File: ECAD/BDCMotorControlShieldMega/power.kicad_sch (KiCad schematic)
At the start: 15 parts, among them Q1 Q_PMOS, Q2 Q_PMOS, Q3 Q_NMOS, Q4 Q_NMOS, Q5 Q_PNP, Q6 Q_PNP, U33 LM2776

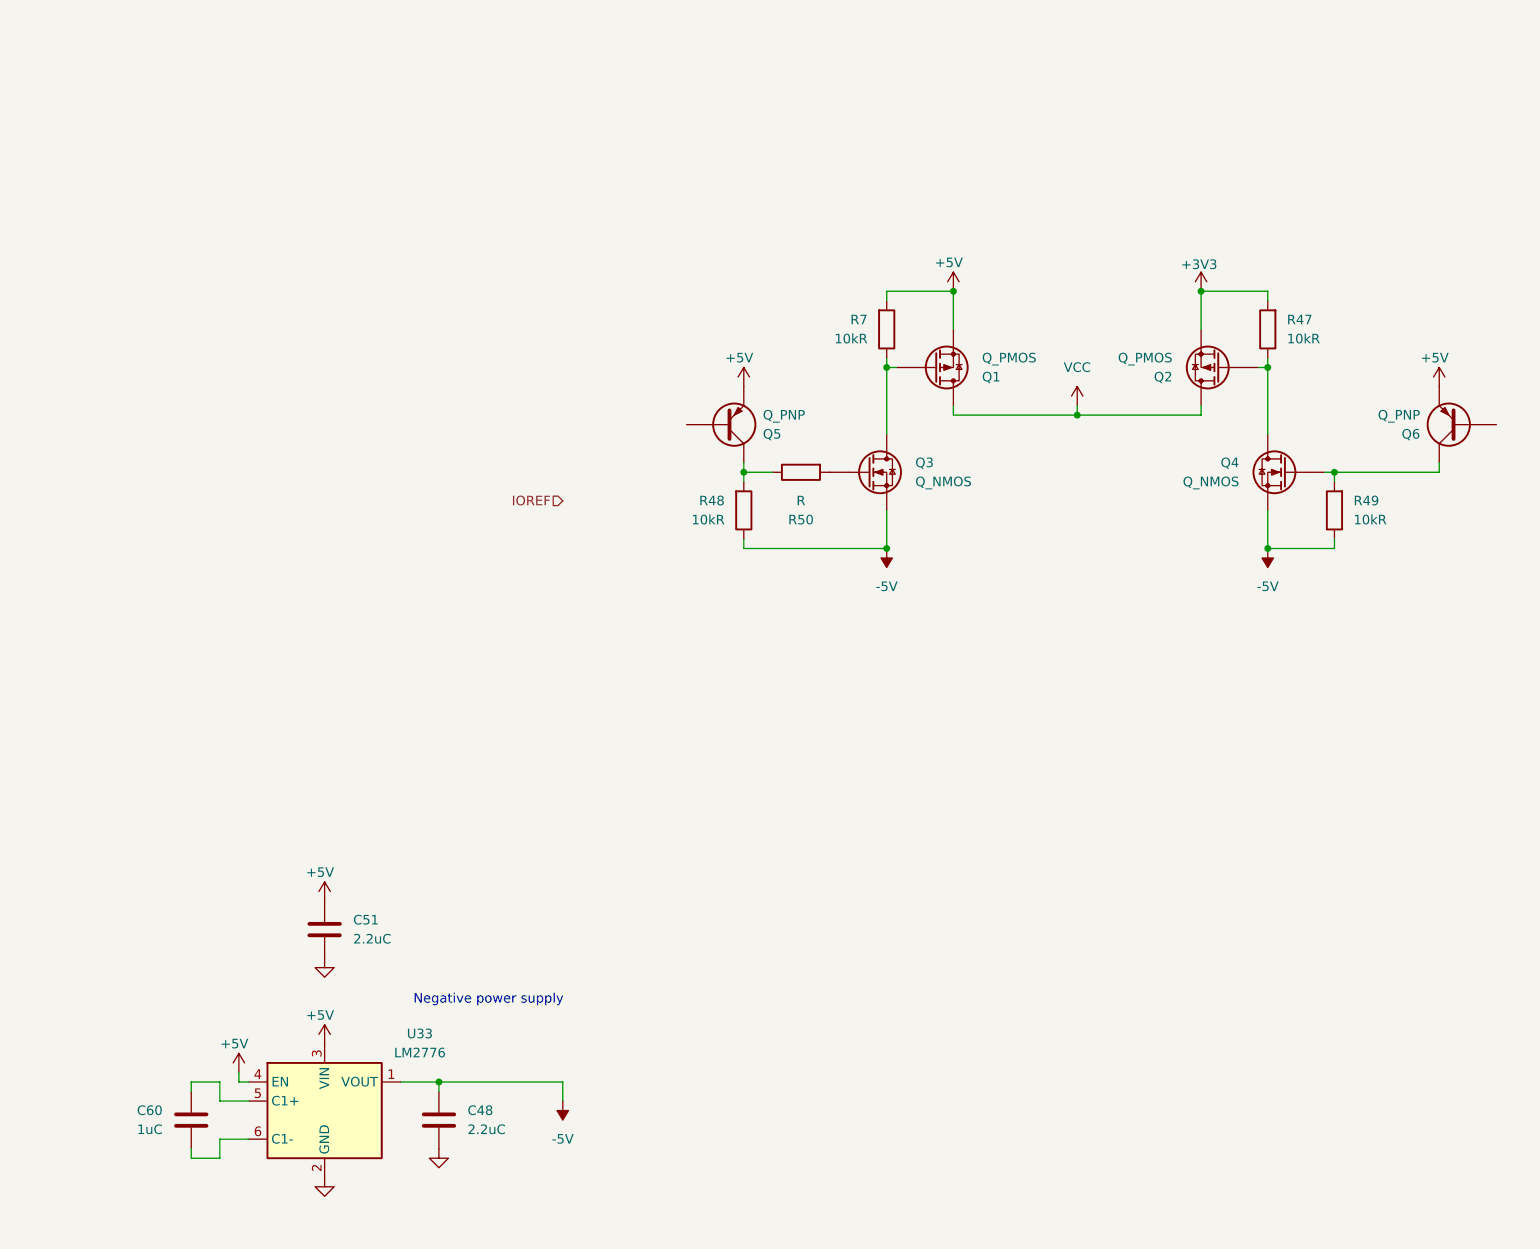
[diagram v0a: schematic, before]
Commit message: Progressed ECAD.
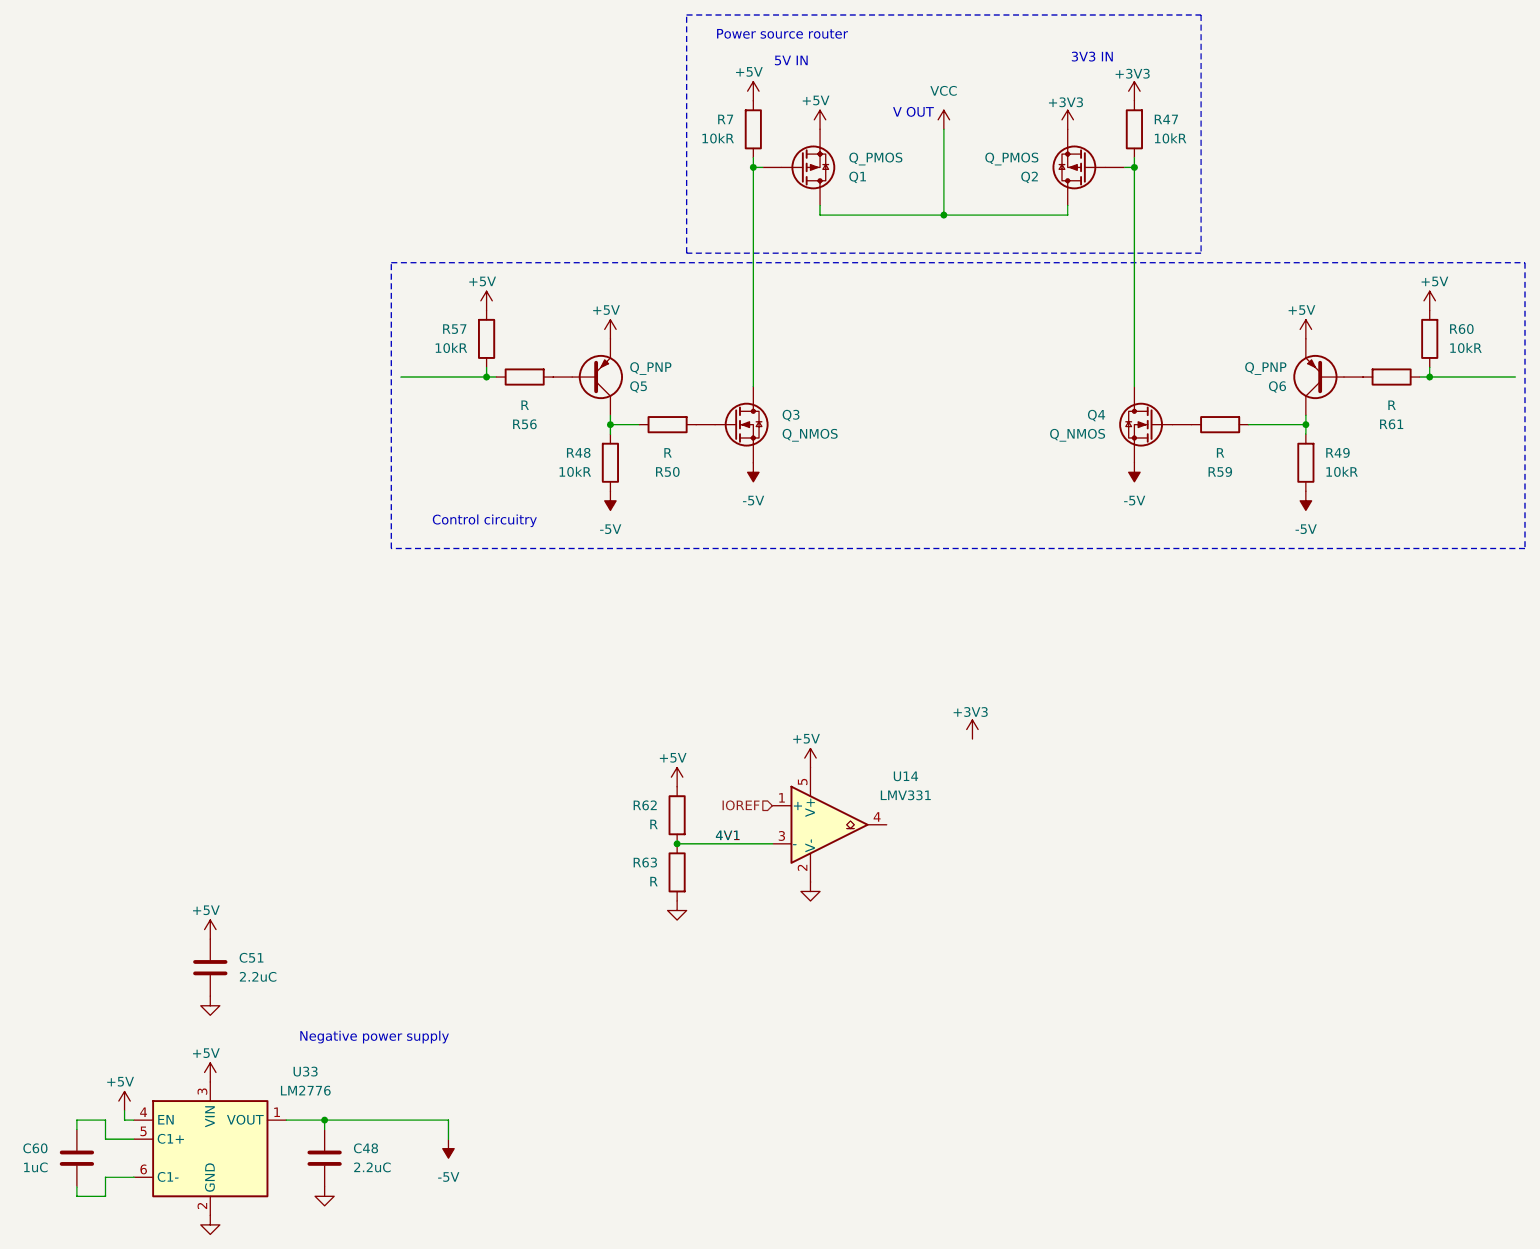
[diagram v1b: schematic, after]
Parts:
- added R56, R59, R61, R62, R63: R, symbol Device:R
- added R57, R60: 10kR, Resistor_SMD:R_0805_2012Metric, symbol Device:R
- added U14: LMV331, symbol Comparator:LMV331
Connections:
- net +5V: now also R57.2, R60.2, R62.1, U14.5 (V+)
- net GND: now also R63.2, U14.2 (V-)
- net IOREF: now also U14.1 (+)
- net at Q6.B: now also R61.2
- net at Q6.C, R49.2: now also R59.2; no longer Q4.G
- net at Q5.B: now also R56.2
- new net: Q4.G, R59.1
- new net: R60.1, R61.1
- new net: R56.1, R57.1
- new net 4V1: R62.2, R63.1, U14.3 (-)
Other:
- note added: "3V3 IN"
- note added: "5V IN"
- note added: "Control circuitry"
- note added: "Power source router"
- note added: "V OUT"
- moved on the sheet: C48, C51, C60, Q1, Q2, Q3, Q4, Q5, Q6, R47, R48, R49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
